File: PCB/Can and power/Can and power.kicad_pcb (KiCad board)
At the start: 2 copper layers, 43.4 x 43.5 mm, 39 parts, among them J1 TPS54232DR, J2 ESP32, J3 12V, J4 C_H, J5 C_L, J6 GND, U1 SN65HVD230

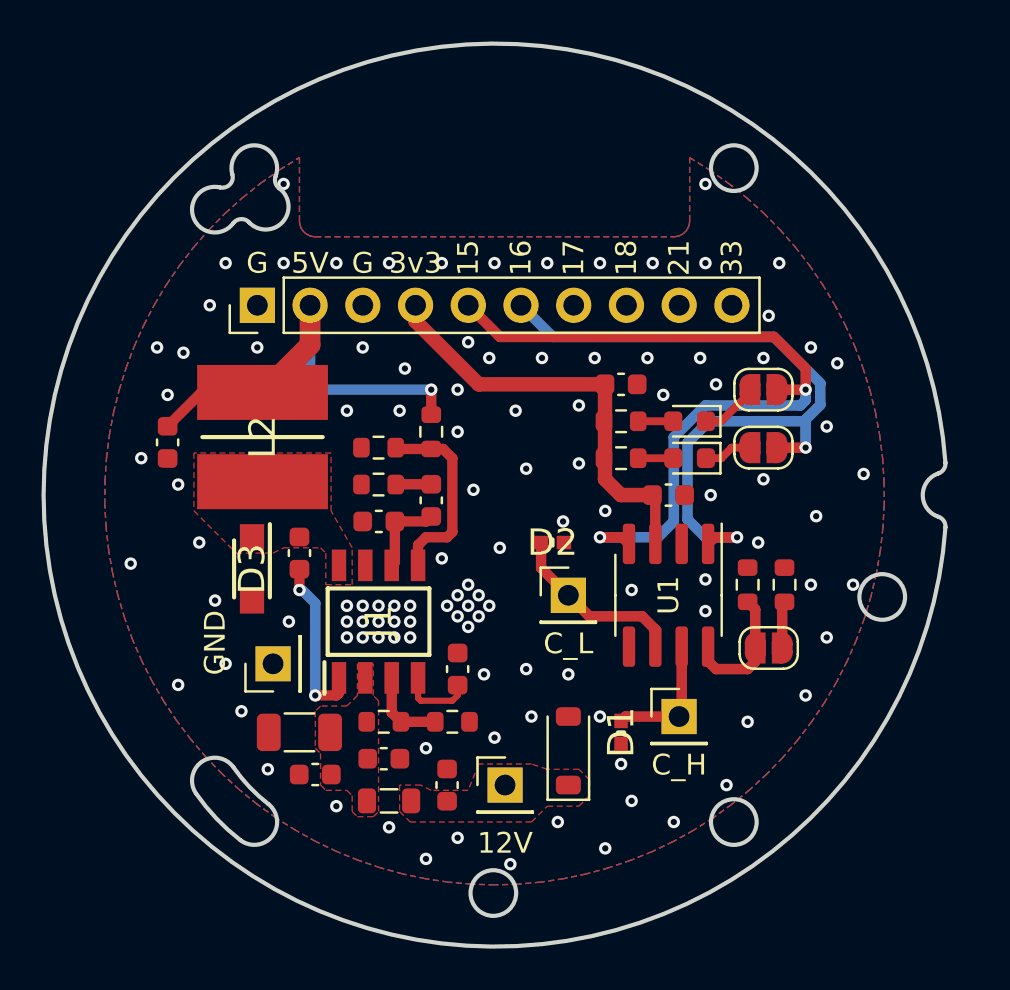
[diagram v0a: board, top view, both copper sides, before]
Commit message: Pre-PCB layout
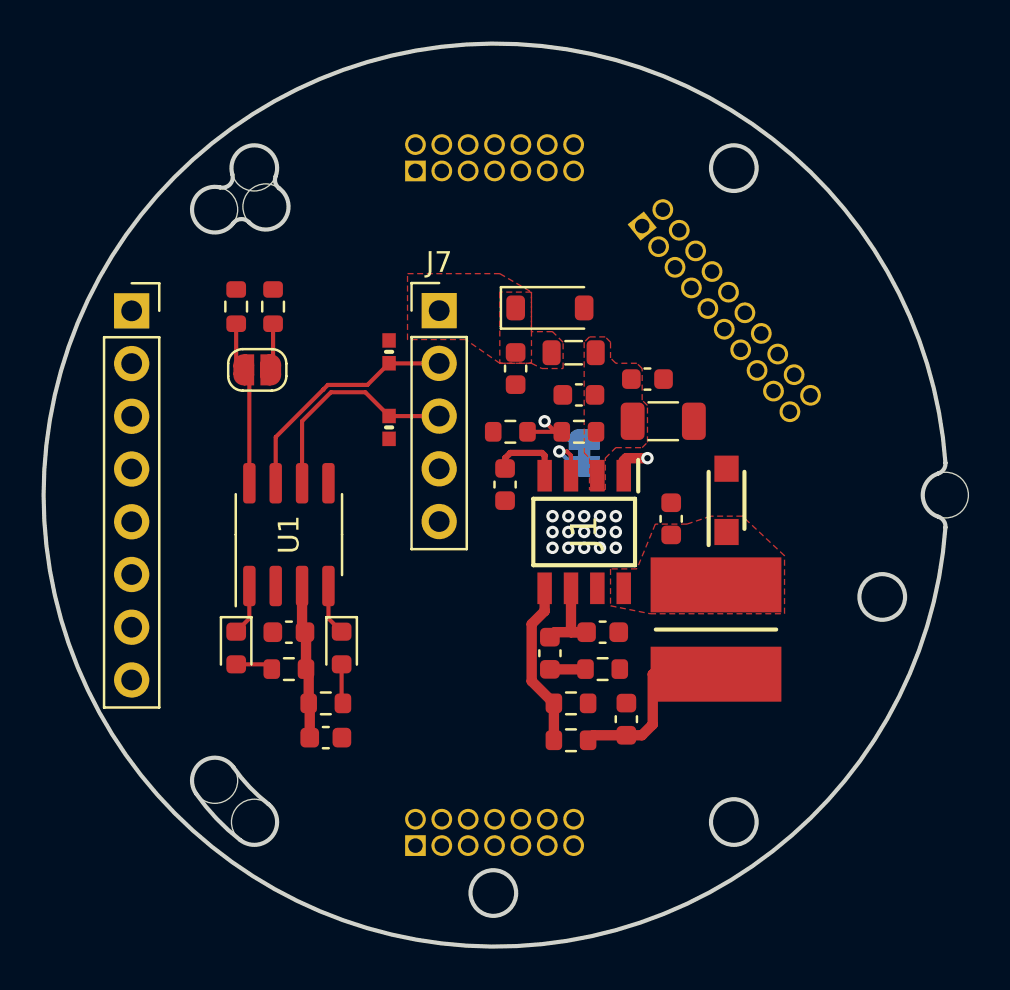
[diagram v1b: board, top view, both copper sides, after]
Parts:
- removed G***: LOGO, Library:QRCode
- removed J2: ESP32, Connector_PinHeader_2.54mm:PinHeader_1x10_P2.54mm_Vertical
- removed JP2, JP3: SolderJumper_2_Open, Jumper:SolderJumper-2_P1.3mm_Open_RoundedPad1.0x1.5mm
- added J7: Car connector, Connector_PinHeader_2.54mm:PinHeader_1x05_P2.54mm_Vertical, F.Cu at (137.3, 91.1)
- added JP4: Use IGN, Jumper:SolderJumper-2_P1.3mm_Bridged_RoundedPad1.0x1.5mm, B.Cu at (144.3, 98.0)
- added REF**: MountingHole_2.2mm_M2, MountingHole:MountingHole_2.2mm_M2, F.Cu at (151.5, 115.8)
- added REF**: MountingHole_2.2mm_M2, MountingHole:MountingHole_2.2mm_M2, F.Cu at (161.7, 100.0)
- added REF**: MountingHole_2.2mm_M2, MountingHole:MountingHole_2.2mm_M2, F.Cu at (129.0, 86.1)
- added REF**: MountingHole_2.2mm_M2, MountingHole:MountingHole_2.2mm_M2, F.Cu at (126.5, 86.2)
- added REF**: MountingHole_2.2mm_M2, MountingHole:MountingHole_2.2mm_M2, F.Cu at (139.9, 119.2)
- added REF**: MountingHole_2.2mm_M2, MountingHole:MountingHole_2.2mm_M2, F.Cu at (128.4, 115.8)
- added REF**: MountingHole_2.2mm_M2, MountingHole:MountingHole_2.2mm_M2, F.Cu at (128.4, 84.2)
- added REF**: MountingHole_2.2mm_M2, MountingHole:MountingHole_2.2mm_M2, F.Cu at (151.5, 84.2)
- added REF**: MountingHole_2.2mm_M2, MountingHole:MountingHole_2.2mm_M2, F.Cu at (126.5, 113.8)
- added REF**: MountingHole_2.2mm_M2, MountingHole:MountingHole_2.2mm_M2, F.Cu at (158.7, 104.9)
- J3: value 12V -> HDR_143_1; footprint Connector_PinHeader_2.54mm:PinHeader_1x01_P2.54mm_Vertical -> Connector_PinSocket_1.27mm:PinSocket_2x07_P1.27mm_Vertical; moved to B.Cu
- J4: value C_H -> HDR_143_2; footprint Connector_PinHeader_2.54mm:PinHeader_1x01_P2.54mm_Vertical -> Connector_PinSocket_1.27mm:PinSocket_2x07_P1.27mm_Vertical; moved to B.Cu
- J5: value C_L -> SKT_146; footprint Connector_PinHeader_2.54mm:PinHeader_1x01_P2.54mm_Vertical -> Connector_PinSocket_1.27mm:PinSocket_2x10_P1.27mm_Vertical; moved to B.Cu
- J6: value GND -> HDR_175; footprint Connector_PinHeader_2.54mm:PinHeader_1x01_P2.54mm_Vertical -> Connector_PinSocket_2.54mm:PinSocket_1x08_P2.54mm_Vertical
- JP1: value SolderJumper_2_Open -> High RS
- moved J4 29.2 mm to (136.2, 84.4), turned to -90 degrees
- moved JP1 28.0 mm to (128.6, 94.0)
- moved R2 28.0 mm to (129.3, 90.9)
- moved R8 28.0 mm to (127.6, 90.9)
- moved C11 25.8 mm to (146.3, 110.8), turned to 90 degrees
- moved C5 24.9 mm to (147.4, 94.4), turned to 0 degrees
- moved L2 23.7 mm to (150.7, 106.5), turned to -90 degrees
- moved D5 23.7 mm to (127.6, 107.4), turned to -90 degrees
- moved FB1 23.3 mm to (143.8, 93.1), turned to 0 degrees
- moved D3 23.1 mm to (151.2, 100.3), turned to 90 degrees
- moved C9 23.1 mm to (148.1, 96.4), turned to 0 degrees
- moved C4 22.2 mm to (131.9, 111.7)
- moved D1 21.5 mm to (134.9, 93.1), turned to 90 degrees
- moved D6 21.4 mm to (142.7, 91.0), turned to 0 degrees
- moved C1 20.3 mm to (141.0, 93.9), turned to 90 degrees
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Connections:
- D1 pad 1: Net-(J4-Pin_1) -> /CAN_H
- D2 pad 1: Net-(J5-Pin_1) -> /CAN_L
- D4 pad 1: Net-(D4-K) -> RX_CAN
- D5 pad 1: Net-(D5-K) -> TX_CAN
- J3 pad 1: +12V -> /143_GPIO0
- J4 pad 1: Net-(J4-Pin_1) -> /143_GPIO45
- J5 pad 1: Net-(J5-Pin_1) -> /146_GPIO13
- J6 pad 1: GND -> /175_GPIO18
- Ren1 pad 1: Net-(J1-EN) -> Net-(JP4-A)
- Ren2 pad 2: Net-(J1-EN) -> Net-(JP4-A)
- U1 pad 1: GPIO16 -> TX_CAN
- U1 pad 4: GPIO15 -> RX_CAN
- U1 pad 6: Net-(J5-Pin_1) -> /CAN_L
- U1 pad 7: Net-(J4-Pin_1) -> /CAN_H
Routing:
- net GPIO15: track 37.0 -> 0.00 mm, vias 2 -> 0
- net GPIO16: track 34.8 -> 0.00 mm, vias 2 -> 0
- net +3V3: track 20.7 -> 7.46 mm
- net VSYS: track 21.4 -> 8.90 mm, vias 1 -> 0
- net /CAN_H: track 0.00 -> 11.6 mm
- net /CAN_L: track 0.00 -> 10.6 mm
- net Net-(J5-Pin_1): track 8.78 -> 0.00 mm
- net Net-(J1-BOOT): track 8.39 -> 1.91 mm, vias 2 -> 1
- net Net-(J4-Pin_1): track 6.30 -> 0.00 mm
- net Net-(JP4-A): track 0.00 -> 4.96 mm, vias 0 -> 1
- net Net-(D4-K): track 2.83 -> 0.00 mm
- net TX_CAN: track 0.00 -> 2.46 mm
- net RX_CAN: track 0.00 -> 2.46 mm
- net Net-(D5-K): track 2.33 -> 0.00 mm
- net Net-(JP1-B): track 6.31 -> 7.95 mm
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- removed copper zone on B.Cu, net GND
- removed copper zone on F.Cu, net GND
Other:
- copper layers 2 -> 4
- board text removed: "15"
- board text removed: "16"
- board text removed: "17"
- board text removed: "18"
- board text removed: "21"
- board text removed: "33"
- board text removed: "3v3"
- board text removed: "5V"
- board text removed: "G"
- board text removed: "MRR"
- board text removed: "WAYWAYWAY"
- board text removed: "rev ${REVISION}"
